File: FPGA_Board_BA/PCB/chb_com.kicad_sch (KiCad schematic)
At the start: 9 parts, among them J12 Box_Header_2x05_THT, J13 Box_Header_2x05_THT, J14 Box_Header_2x05_THT, J15 Box_Header_2x05_THT, J18 Plug_Terminal_2x12pin, U26 BoxHeader_24pin, U45 BoxHeader_24pin, U46 BoxHeader_24pin, U47 BoxHeader_24pin

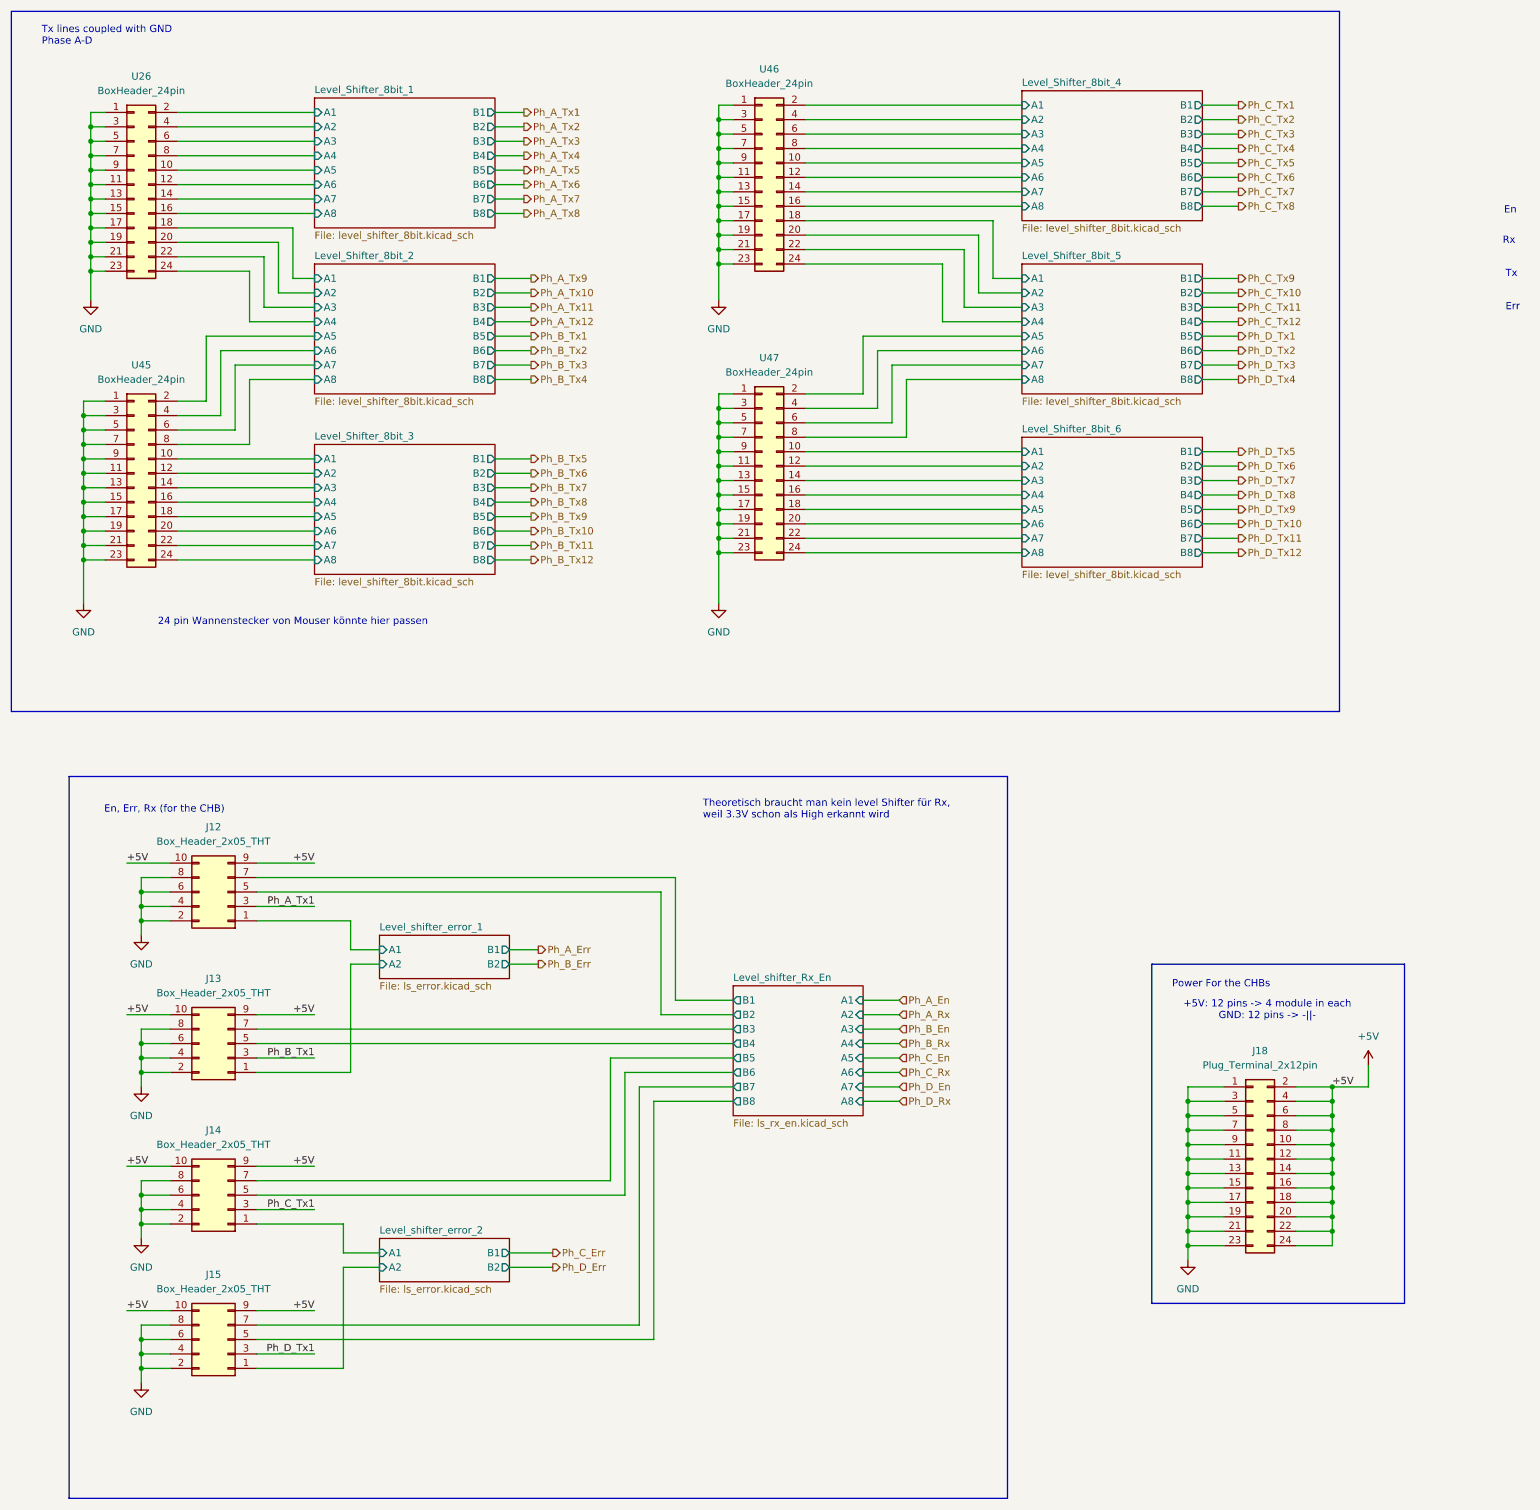
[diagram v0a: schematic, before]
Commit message: right side almost finished
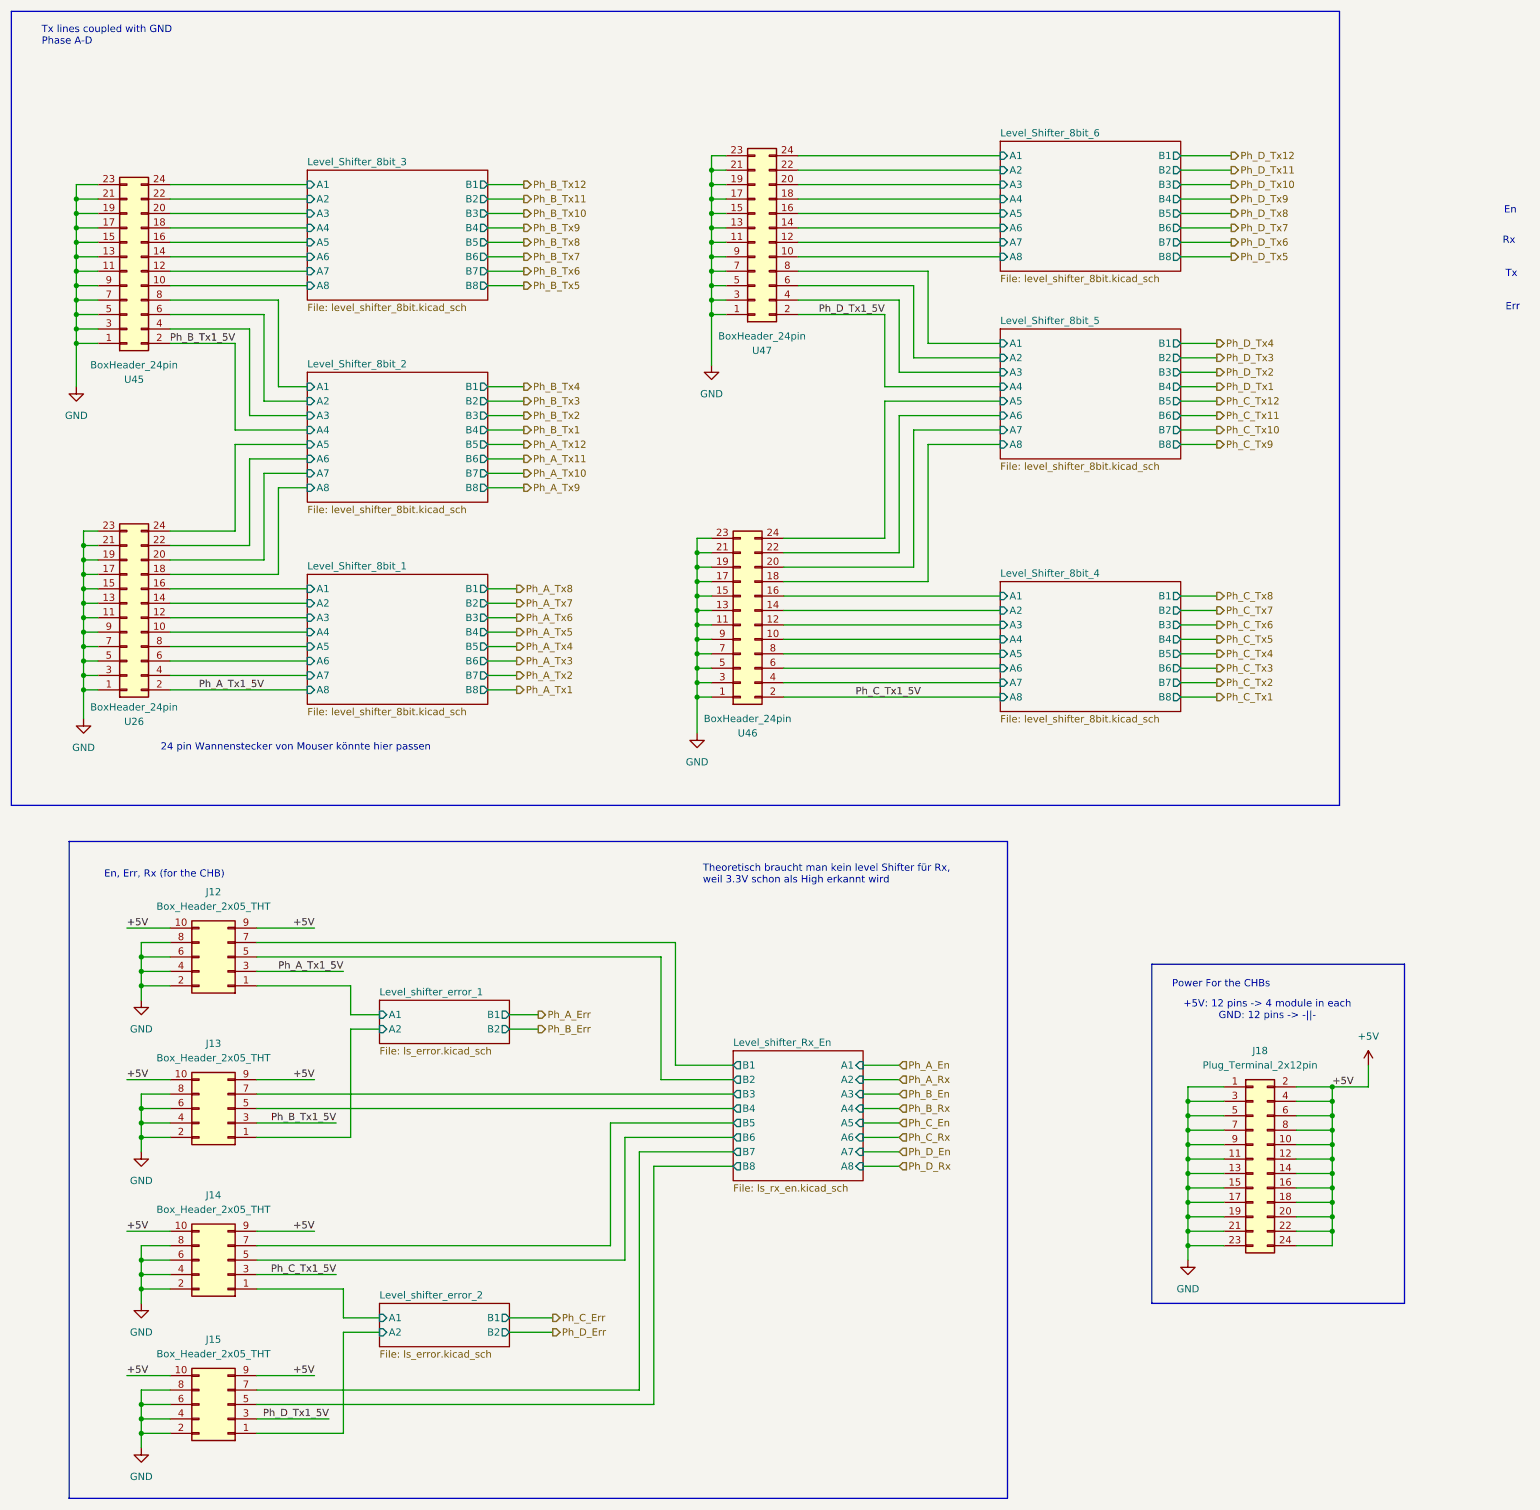
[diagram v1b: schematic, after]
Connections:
- net Level_Shifter_8bit_1/A8 is gone; now on net Level_Shifter_8bit_1/A1: U26.16
- net Level_Shifter_8bit_2/A4 is gone; now on net Level_Shifter_8bit_2/A5: U26.24
- net Level_Shifter_8bit_4/A8 is gone; now on net Level_Shifter_8bit_4/A1: U46.16
- net Level_Shifter_8bit_5/A4 is gone; now on net Level_Shifter_8bit_5/A5: U46.24
- net Level_Shifter_8bit_1/A1: no longer U26.2
- net Level_Shifter_8bit_1/A2: now also U26.14; no longer U26.4
- net Level_Shifter_8bit_1/A3: now also U26.12; no longer U26.6
- net Level_Shifter_8bit_1/A4: now also U26.10; no longer U26.8
- net Level_Shifter_8bit_1/A5: now also U26.8; no longer U26.10
- net Level_Shifter_8bit_1/A6: now also U26.6; no longer U26.12
- net Level_Shifter_8bit_1/A7: now also U26.4; no longer U26.14
- net Level_Shifter_8bit_2/A1: now also U45.8; no longer U26.18
- net Level_Shifter_8bit_2/A2: now also U45.6; no longer U26.20
- net Level_Shifter_8bit_2/A3: now also U45.4; no longer U26.22
- net Level_Shifter_8bit_2/A5: no longer U45.2
- net Level_Shifter_8bit_2/A6: now also U26.22; no longer U45.4
- net Level_Shifter_8bit_2/A7: now also U26.20; no longer U45.6
- net Level_Shifter_8bit_2/A8: now also U26.18; no longer U45.8
- net Level_Shifter_8bit_3/A1: now also U45.24; no longer U45.10
- net Level_Shifter_8bit_3/A2: now also U45.22; no longer U45.12
- net Level_Shifter_8bit_3/A3: now also U45.20; no longer U45.14
- net Level_Shifter_8bit_3/A4: now also U45.18; no longer U45.16
- net Level_Shifter_8bit_3/A5: now also U45.16; no longer U45.18
- net Level_Shifter_8bit_3/A6: now also U45.14; no longer U45.20
- net Level_Shifter_8bit_3/A7: now also U45.12; no longer U45.22
- net Level_Shifter_8bit_3/A8: now also U45.10; no longer U45.24
- net Level_Shifter_8bit_4/A1: no longer U46.2
- net Level_Shifter_8bit_4/A2: now also U46.14; no longer U46.4
- net Level_Shifter_8bit_4/A3: now also U46.12; no longer U46.6
- net Level_Shifter_8bit_4/A4: now also U46.10; no longer U46.8
- net Level_Shifter_8bit_4/A5: now also U46.8; no longer U46.10
- net Level_Shifter_8bit_4/A6: now also U46.6; no longer U46.12
- net Level_Shifter_8bit_4/A7: now also U46.4; no longer U46.14
- net Level_Shifter_8bit_5/A1: now also U47.8; no longer U46.18
- net Level_Shifter_8bit_5/A2: now also U47.6; no longer U46.20
- net Level_Shifter_8bit_5/A3: now also U47.4; no longer U46.22
- net Level_Shifter_8bit_5/A5: no longer U47.2
- net Level_Shifter_8bit_5/A6: now also U46.22; no longer U47.4
- net Level_Shifter_8bit_5/A7: now also U46.20; no longer U47.6
- net Level_Shifter_8bit_5/A8: now also U46.18; no longer U47.8
- net Level_Shifter_8bit_6/A1: now also U47.24; no longer U47.10
- net Level_Shifter_8bit_6/A2: now also U47.22; no longer U47.12
- net Level_Shifter_8bit_6/A3: now also U47.20; no longer U47.14
- net Level_Shifter_8bit_6/A4: now also U47.18; no longer U47.16
- net Level_Shifter_8bit_6/A5: now also U47.16; no longer U47.18
- net Level_Shifter_8bit_6/A6: now also U47.14; no longer U47.20
- net Level_Shifter_8bit_6/A7: now also U47.12; no longer U47.22
- net Level_Shifter_8bit_6/A8: now also U47.10; no longer U47.24
- net Ph_A_Tx1: no longer J12.3 (Pin_3)
- net Ph_B_Tx1: no longer J13.3 (Pin_3)
- net Ph_C_Tx1: no longer J14.3 (Pin_3)
- net Ph_D_Tx1: no longer J15.3 (Pin_3)
- new net Ph_A_Tx1_5V: J12.3 (Pin_3), U26.2
- new net Ph_B_Tx1_5V: J13.3 (Pin_3), U45.2
- new net Ph_C_Tx1_5V: J14.3 (Pin_3), U46.2
- new net Ph_D_Tx1_5V: J15.3 (Pin_3), U47.2
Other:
- moved on the sheet: J12, J13, J14, J15, U26, U45, U46, U47
